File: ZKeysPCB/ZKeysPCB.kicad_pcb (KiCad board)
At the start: 2 copper layers, 73.7 x 50.8 mm, 15 parts, among them SW1 SW_Push, SW2 SW_Push, SW3 SW_Push, SW4 SW_Push, SW5 SW_Push, SW6 SW_Push, U1 Teensy-LC

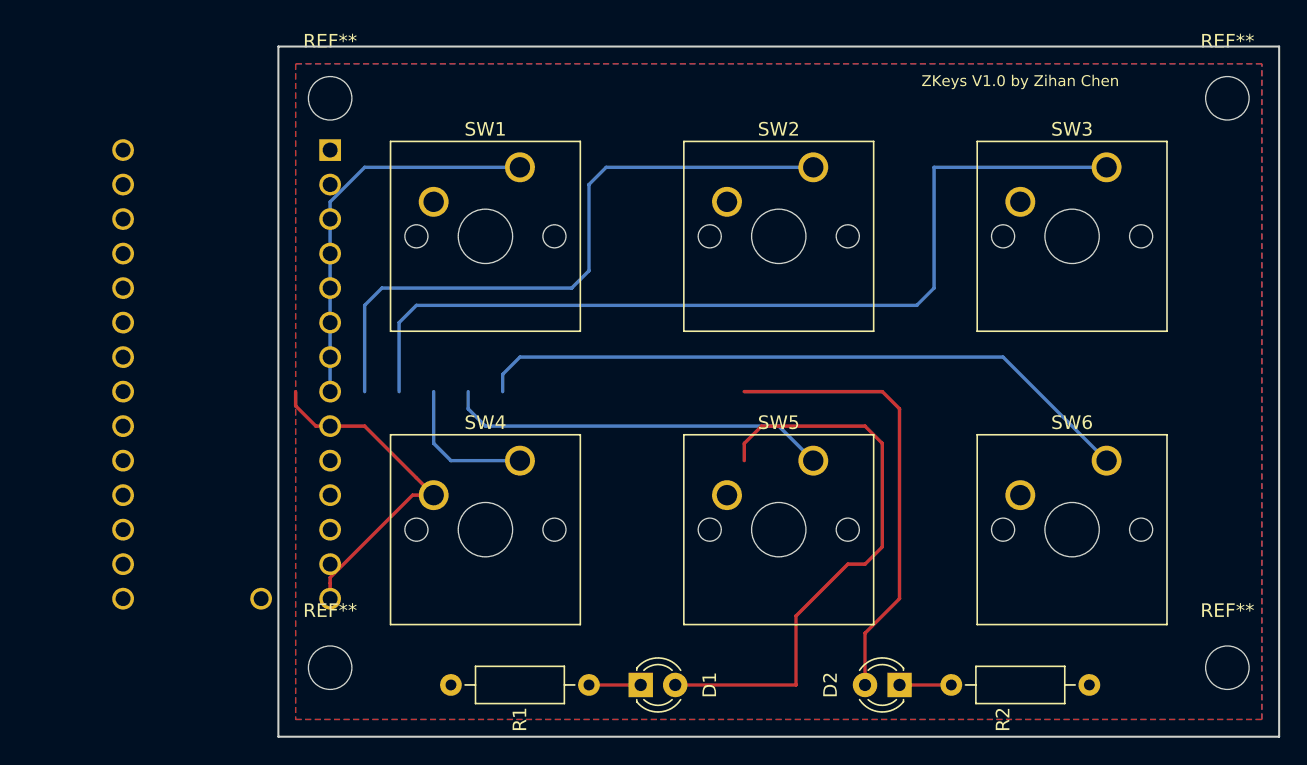
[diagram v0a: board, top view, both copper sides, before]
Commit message: updated PCB drawing
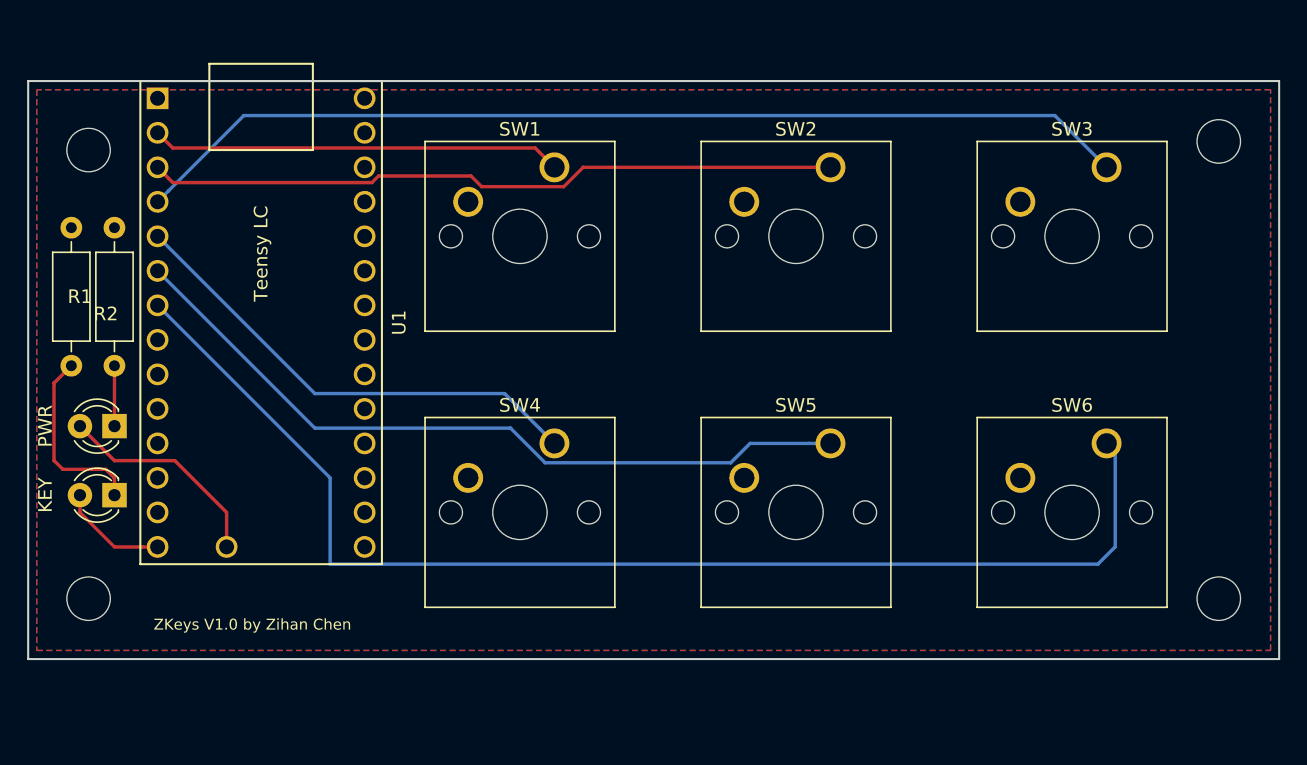
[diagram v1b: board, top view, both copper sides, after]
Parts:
- removed the REF** at (87.6, 90.2)
- removed the REF** at (87.6, 132.1)
- removed the REF** at (153.7, 132.1)
- added REF**: MountingHole_3.2mm_M3, MountingHole:MountingHole_3.2mm_M3, F.Cu at (69.8, 127.0)
- added REF**: MountingHole_3.2mm_M3, MountingHole:MountingHole_3.2mm_M3, F.Cu at (69.8, 94.0)
- added REF**: MountingHole_3.2mm_M3, MountingHole:MountingHole_3.2mm_M3, F.Cu at (153.0, 127.0)
- U1: moved to F.Cu
- moved R2 68.9 mm to (68.6, 109.9), turned to 90 degrees
- moved KEY 59.4 mm to (71.8, 119.4)
- moved PWR 43.2 mm to (71.8, 114.3), turned to 180 degrees
- moved R1 42.1 mm to (71.8, 109.9), turned to 90 degrees
- moved U1 4.58 mm to (82.5, 106.7)
- moved REF** 3.24 mm to (153.0, 93.3)
- moved SW4 2.84 mm to (104.1, 115.6)
- moved SW1 2.54 mm to (104.1, 95.2)
- moved SW5 1.80 mm to (124.5, 115.6)
- moved SW6 1.27 mm to (144.8, 115.6)
- moved SW2 1.27 mm to (124.5, 95.2)
- renumbered D2 to KEY, D1 to PWR
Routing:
- net BTN_INC: track 49.4 -> 90.5 mm
- net BTN_DEC: track 28.2 -> 56.0 mm
- net Net-(D1-Pad2): track 42.5 -> 16.0 mm
- net GND: track 25.6 -> 0.00 mm
- net Net-(D2-Pad2): track 33.3 -> 8.04 mm
- net BTN_MUTE: track 10.7 -> 35.5 mm
- net Net-(D2-Pad1): track 3.81 -> 13.8 mm
- net BTN_NEXT: track 67.1 -> 74.1 mm
- net BTN_PLAY: track 47.3 -> 51.1 mm
- net BTN_PREV: track 29.0 -> 30.3 mm
- net Net-(D1-Pad1): track 3.81 -> 4.44 mm
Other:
- board size 73.7 x 50.8 mm -> 92.1 x 42.5 mm
